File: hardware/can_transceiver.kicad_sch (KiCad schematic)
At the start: 5 parts, among them U7 MCP2562-H-SN

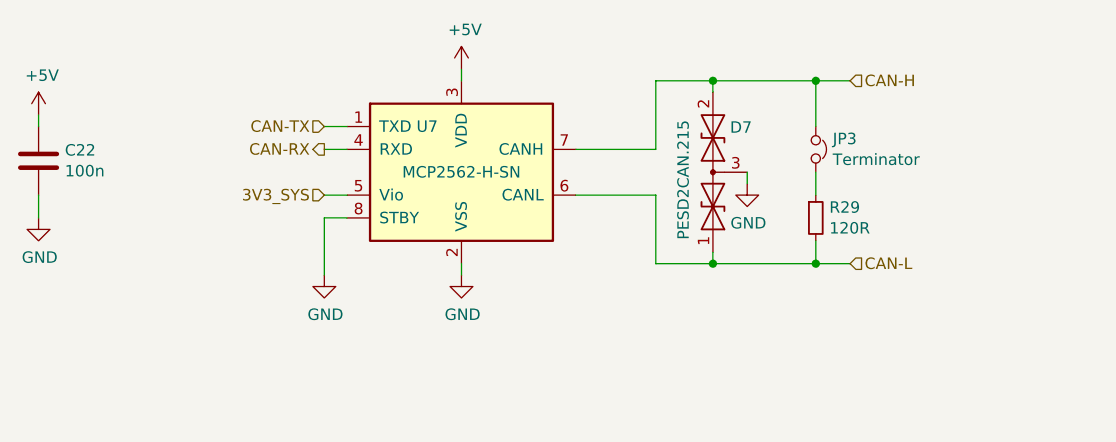
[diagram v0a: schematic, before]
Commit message: Refactor
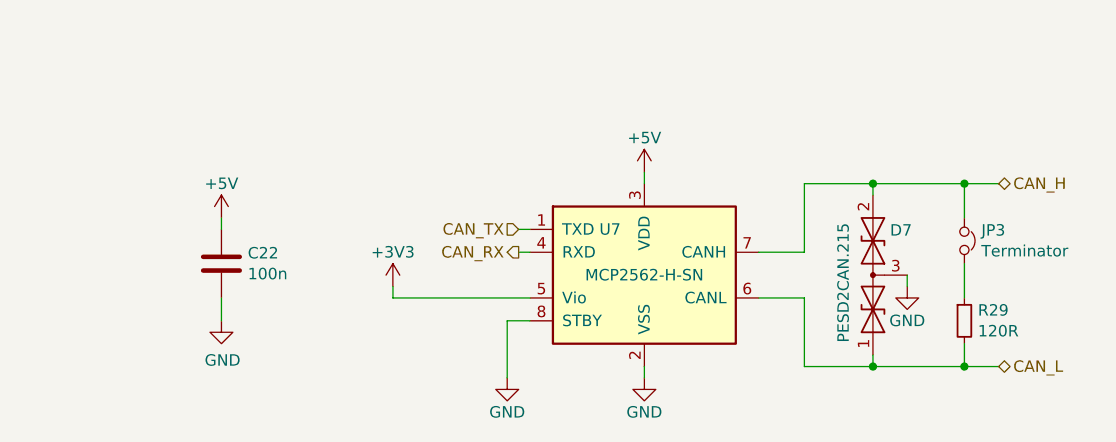
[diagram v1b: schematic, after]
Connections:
- net 3V3_SYS renamed +3V3
- net CAN-H renamed CAN_H
- net CAN-L renamed CAN_L
- net CAN-RX renamed CAN_RX
- net CAN-TX renamed CAN_TX
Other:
- title: CAN Communication -> CAN Transceiver
- moved on the sheet: C22, D7, JP3, R29, U7
